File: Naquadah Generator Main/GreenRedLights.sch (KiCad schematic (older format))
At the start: 2 parts, among them J4 Conn_01x02, J5 Conn_01x02

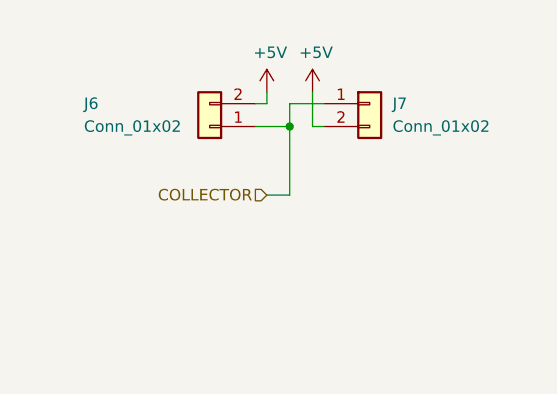
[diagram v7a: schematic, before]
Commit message: Updates
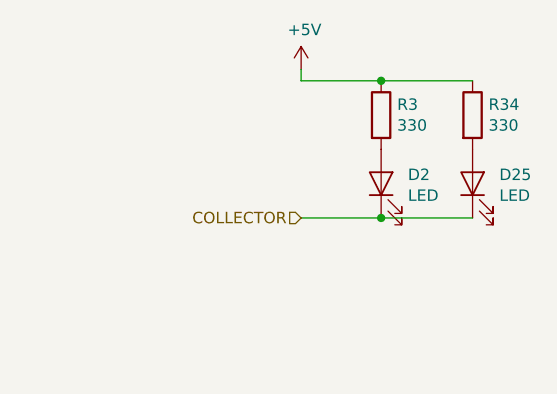
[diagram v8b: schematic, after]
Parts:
- removed J4, J5: Conn_01x02, Connector_Wire:SolderWirePad_1x02_P3.81mm_Drill1.2mm, symbol Connector_Generic:Conn_01x02
- added D2, D25: LED, LED_SMD:LED_1812_4532Metric, symbol Device:LED
- added R3, R34: 330, Frequently_Used:0805_2012Metric_HandSolder, symbol Device:R
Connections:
- net +5V: now also R3.1, R34.1
- net COLLECTOR: now also D2.1 (K), D25.1 (K)
- new net: D2.2 (A), R3.2
- new net: D25.2 (A), R34.2
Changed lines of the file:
@@
 $Descr A4 11693 8268
 encoding utf-8
-Sheet 10 11
+Sheet 8 11
 Title ""
 Date ""
@@
 Comment4 ""
 $EndDescr
+Text HLabel 5500 4250 0    50   Input ~ 0
+COLLECTOR
 Wire Wire Line
-	5350 4150 5450 4150
-Text HLabel 5350 4150 0    50   Input ~ 0
-COLLECTOR
+	5500 4250 5850 4250
+Connection ~ 5850 4250
 $Comp
-L Connector_Generic:Conn_01x02 J?
-U 1 1 5EAB251D
-P 5800 3750
-AR Path="/5EA45E37/5EAB251D" Ref="J?"  Part="1"
-AR Path="/5EA4676F/5EAB251D" Ref="J?"  Part="1"
-AR Path="/5EA46A2B/5EAB251D" Ref="J?"  Part="1"
-AR Path="/5ED17BA0/5ED2A32F/5EAB251D" Ref="J5"  Part="1"
-AR Path="/5ED17BA0/5ED2A36D/5EAB251D" Ref="J7"  Part="1"
-F 0 "J7" H 5900 3750 50  0000 L CNN
-F 1 "Conn_01x02" H 5900 3650 50  0000 L CNN
-F 2 "Connector_Wire:SolderWirePad_1x02_P3.81mm_Drill1.2mm" H 5800 3750 50  0001 C CNN
-F 3 "~" H 5800 3750 50  0001 C CNN
-	1    5800 3750
+L Device:LED D?
+U 1 1 5EEF3073
+P 5850 4100
+AR Path="/5E9E5DDE/5EEF3073" Ref="D?"  Part="1"
+AR Path="/5E9E304D/5EEF3073" Ref="D?"  Part="1"
+AR Path="/5E9D240B/5EEF3073" Ref="D?"  Part="1"
+AR Path="/5E9E5DE1/5EEF3073" Ref="D?"  Part="1"
+AR Path="/5E9E4A6B/5EEF3073" Ref="D?"  Part="1"
+AR Path="/5ED17BA0/5ED2A301/5EEF3073" Ref="D?"  Part="1"
+AR Path="/5ED17BA0/5ED2A304/5EEF3073" Ref="D?"  Part="1"
+AR Path="/5ED17BA0/5ED2A307/5EEF3073" Ref="D?"  Part="1"
+AR Path="/5ED17BA0/5ED2A30A/5EEF3073" Ref="D?"  Part="1"
+AR Path="/5ED17BA0/5ED2A30D/5EEF3073" Ref="D?"  Part="1"
+AR Path="/5ED17BA0/5ED2A32F/5EEF3073" Ref="D2"  Part="1"
+AR Path="/5ED17BA0/5ED2A36D/5EEF3073" Ref="D26"  Part="1"
+F 0 "D2" V 5889 3983 50  0000 R CNN
+F 1 "LED" V 5798 3983 50  0000 R CNN
+F 2 "LED_SMD:LED_1812_4532Metric" H 5850 4100 50  0001 C CNN
+F 3 "~" H 5850 4100 50  0001 C CNN
+	1    5850 4100
+	0    -1   -1   0
+$EndComp
+Wire Wire Line
+	5850 3650 5500 3650
+Connection ~ 5850 3650
+$Comp
+L Device:R R?
+U 1 1 5EEF307B
+P 5850 3800
+AR Path="/5E9E5DDE/5EEF307B" Ref="R?"  Part="1"
+AR Path="/5E9E304D/5EEF307B" Ref="R?"  Part="1"
+AR Path="/5E9D240B/5EEF307B" Ref="R?"  Part="1"
+AR Path="/5E9E5DE1/5EEF307B" Ref="R?"  Part="1"
+AR Path="/5E9E4A6B/5EEF307B" Ref="R?"  Part="1"
+AR Path="/5ED17BA0/5ED2A301/5EEF307B" Ref="R?"  Part="1"
+AR Path="/5ED17BA0/5ED2A304/5EEF307B" Ref="R?"  Part="1"
+AR Path="/5ED17BA0/5ED2A307/5EEF307B" Ref="R?"  Part="1"
+AR Path="/5ED17BA0/5ED2A30A/5EEF307B" Ref="R?"  Part="1"
+AR Path="/5ED17BA0/5ED2A30D/5EEF307B" Ref="R?"  Part="1"
+AR Path="/5ED17BA0/5ED2A32F/5EEF307B" Ref="R3"  Part="1"
+AR Path="/5ED17BA0/5ED2A36D/5EEF307B" Ref="R35"  Part="1"
+F 0 "R3" H 5920 3846 50  0000 L CNN
+F 1 "330" H 5920 3755 50  0000 L CNN
+F 2 "Frequently_Used:0805_2012Metric_HandSolder" V 5780 3800 50  0001 C CNN
+F 3 "~" H 5850 3800 50  0001 C CNN
+	1    5850 3800
 	1    0    0    -1
 $EndComp
+Wire Wire Line
+	5850 3650 6250 3650
 $Comp
-L Connector_Generic:Conn_01x02 J?
-U 1 1 5EA51394
-P 5100 3850
-AR Path="/5EA45E37/5EA51394" Ref="J?"  Part="1"
-AR Path="/5EA4676F/5EA51394" Ref="J?"  Part="1"
-AR Path="/5EA46A2B/5EA51394" Ref="J?"  Part="1"
-AR Path="/5ED17BA0/5ED2A32F/5EA51394" Ref="J4"  Part="1"
-AR Path="/5ED17BA0/5ED2A36D/5EA51394" Ref="J6"  Part="1"
-F 0 "J6" H 5650 3750 50  0000 R CNN
-F 1 "Conn_01x02" H 5650 3850 50  0000 R CNN
-F 2 "Connector_Wire:SolderWirePad_1x02_P3.81mm_Drill1.2mm" H 5100 3850 50  0001 C CNN
-F 3 "~" H 5100 3850 50  0001 C CNN
-	1    5100 3850
-	-1   0    0    1
+L Device:R R?
+U 1 1 5EEF3083
+P 6250 3800
+AR Path="/5E9E5DDE/5EEF3083" Ref="R?"  Part="1"
+AR Path="/5E9E304D/5EEF3083" Ref="R?"  Part="1"
+AR Path="/5E9D240B/5EEF3083" Ref="R?"  Part="1"
+AR Path="/5E9E5DE1/5EEF3083" Ref="R?"  Part="1"
+AR Path="/5E9E4A6B/5EEF3083" Ref="R?"  Part="1"
+AR Path="/5ED17BA0/5ED2A301/5EEF3083" Ref="R?"  Part="1"
+AR Path="/5ED17BA0/5ED2A304/5EEF3083" Ref="R?"  Part="1"
+AR Path="/5ED17BA0/5ED2A307/5EEF3083" Ref="R?"  Part="1"
+AR Path="/5ED17BA0/5ED2A30A/5EEF3083" Ref="R?"  Part="1"
+AR Path="/5ED17BA0/5ED2A30D/5EEF3083" Ref="R?"  Part="1"
+AR Path="/5ED17BA0/5ED2A32F/5EEF3083" Ref="R34"  Part="1"
+AR Path="/5ED17BA0/5ED2A36D/5EEF3083" Ref="R36"  Part="1"
+F 0 "R34" H 6320 3846 50  0000 L CNN
+F 1 "330" H 6320 3755 50  0000 L CNN
+F 2 "Frequently_Used:0805_2012Metric_HandSolder" V 6180 3800 50  0001 C CNN
+F 3 "~" H 6250 3800 50  0001 C CNN
+	1    6250 3800
+	1    0    0    -1
 $EndComp
 Wire Wire Line
-	5600 3750 5450 3750
-Wire Wire Line
-	5450 3750 5450 3850
-Wire Wire Line
-	5300 3850 5450 3850
-Connection ~ 5450 3850
-Wire Wire Line
-	5450 3850 5450 4150
-Wire Wire Line
-	5350 3700 5350 3750
-Wire Wire Line
-	5600 3850 5550 3850
-Wire Wire Line
-	5550 3850 5550 3700
+	5850 4250 6250 4250
 $Comp
-L power:+5V #PWR?
-U 1 1 5EC1DBF9
-P 5350 3700
-AR Path="/5EA45E37/5EC1DBF9" Ref="#PWR?"  Part="1"
-AR Path="/5EA4676F/5EC1DBF9" Ref="#PWR?"  Part="1"
-AR Path="/5ED17BA0/5ED2A32F/5EC1DBF9" Ref="#PWR046"  Part="1"
-AR Path="/5ED17BA0/5ED2A36D/5EC1DBF9" Ref="#PWR049"  Part="1"
-F 0 "#PWR049" H 5350 3550 50  0001 C CNN
-F 1 "+5V" H 5365 3873 50  0000 C CNN
-F 2 "" H 5350 3700 50  0001 C CNN
-F 3 "" H 5350 3700 50  0001 C CNN
-	1    5350 3700
-	1    0    0    -1
+L Device:LED D?
+U 1 1 5EEF308D
+P 6250 4100
+AR Path="/5E9E5DDE/5EEF308D" Ref="D?"  Part="1"
+AR Path="/5E9E304D/5EEF308D" Ref="D?"  Part="1"
+AR Path="/5E9D240B/5EEF308D" Ref="D?"  Part="1"
+AR Path="/5E9E5DE1/5EEF308D" Ref="D?"  Part="1"
+AR Path="/5E9E4A6B/5EEF308D" Ref="D?"  Part="1"
+AR Path="/5ED17BA0/5ED2A301/5EEF308D" Ref="D?"  Part="1"
+AR Path="/5ED17BA0/5ED2A304/5EEF308D" Ref="D?"  Part="1"
+AR Path="/5ED17BA0/5ED2A307/5EEF308D" Ref="D?"  Part="1"
+AR Path="/5ED17BA0/5ED2A30A/5EEF308D" Ref="D?"  Part="1"
+AR Path="/5ED17BA0/5ED2A30D/5EEF308D" Ref="D?"  Part="1"
+AR Path="/5ED17BA0/5ED2A32F/5EEF308D" Ref="D25"  Part="1"
+AR Path="/5ED17BA0/5ED2A36D/5EEF308D" Ref="D27"  Part="1"
+F 0 "D25" V 6289 3983 50  0000 R CNN
+F 1 "LED" V 6198 3983 50  0000 R CNN
+F 2 "LED_SMD:LED_1812_4532Metric" H 6250 4100 50  0001 C CNN
+F 3 "~" H 6250 4100 50  0001 C CNN
+	1    6250 4100
+	0    -1   -1   0
 $EndComp
 $Comp
 L power:+5V #PWR?
-U 1 1 5EC1E71E
-P 5550 3700
-AR Path="/5EA45E37/5EC1E71E" Ref="#PWR?"  Part="1"
-AR Path="/5EA4676F/5EC1E71E" Ref="#PWR?"  Part="1"
-AR Path="/5ED17BA0/5ED2A32F/5EC1E71E" Ref="#PWR048"  Part="1"
-AR Path="/5ED17BA0/5ED2A36D/5EC1E71E" Ref="#PWR051"  Part="1"
-F 0 "#PWR051" H 5550 3550 50  0001 C CNN
-F 1 "+5V" H 5565 3873 50  0000 C CNN
-F 2 "" H 5550 3700 50  0001 C CNN
-F 3 "" H 5550 3700 50  0001 C CNN
-	1    5550 3700
+U 1 1 5EEF3093
+P 5500 3600
+AR Path="/5E9E304D/5EEF3093" Ref="#PWR?"  Part="1"
+AR Path="/5E9E5DE1/5EEF3093" Ref="#PWR?"  Part="1"
+AR Path="/5E9E5DDE/5EEF3093" Ref="#PWR?"  Part="1"
+AR Path="/5E9E4A6B/5EEF3093" Ref="#PWR?"  Part="1"
+AR Path="/5E9D240B/5EEF3093" Ref="#PWR?"  Part="1"
+AR Path="/5ED17BA0/5ED2A301/5EEF3093" Ref="#PWR?"  Part="1"
+AR Path="/5ED17BA0/5ED2A304/5EEF3093" Ref="#PWR?"  Part="1"
+AR Path="/5ED17BA0/5ED2A307/5EEF3093" Ref="#PWR?"  Part="1"
+AR Path="/5ED17BA0/5ED2A30A/5EEF3093" Ref="#PWR?"  Part="1"
+AR Path="/5ED17BA0/5ED2A30D/5EEF3093" Ref="#PWR?"  Part="1"
+AR Path="/5ED17BA0/5ED2A32F/5EEF3093" Ref="#PWR012"  Part="1"
+AR Path="/5ED17BA0/5ED2A36D/5EEF3093" Ref="#PWR013"  Part="1"
+F 0 "#PWR013" H 5500 3450 50  0001 C CNN
+F 1 "+5V" H 5515 3773 50  0000 C CNN
+F 2 "" H 5500 3600 50  0001 C CNN
+F 3 "" H 5500 3600 50  0001 C CNN
+	1    5500 3600
 	1    0    0    -1
 $EndComp
 Wire Wire Line
-	5350 3750 5300 3750
+	5500 3600 5500 3650
 $EndSCHEMATC
